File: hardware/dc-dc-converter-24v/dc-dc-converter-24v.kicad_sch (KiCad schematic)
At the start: 56 parts, among them J1 12V, J2 24V, Q1 SQJA42EP, Q2 SQJA42EP, Q3 SQJA42EP, Q4 SQJA42EP, U1 LM5176

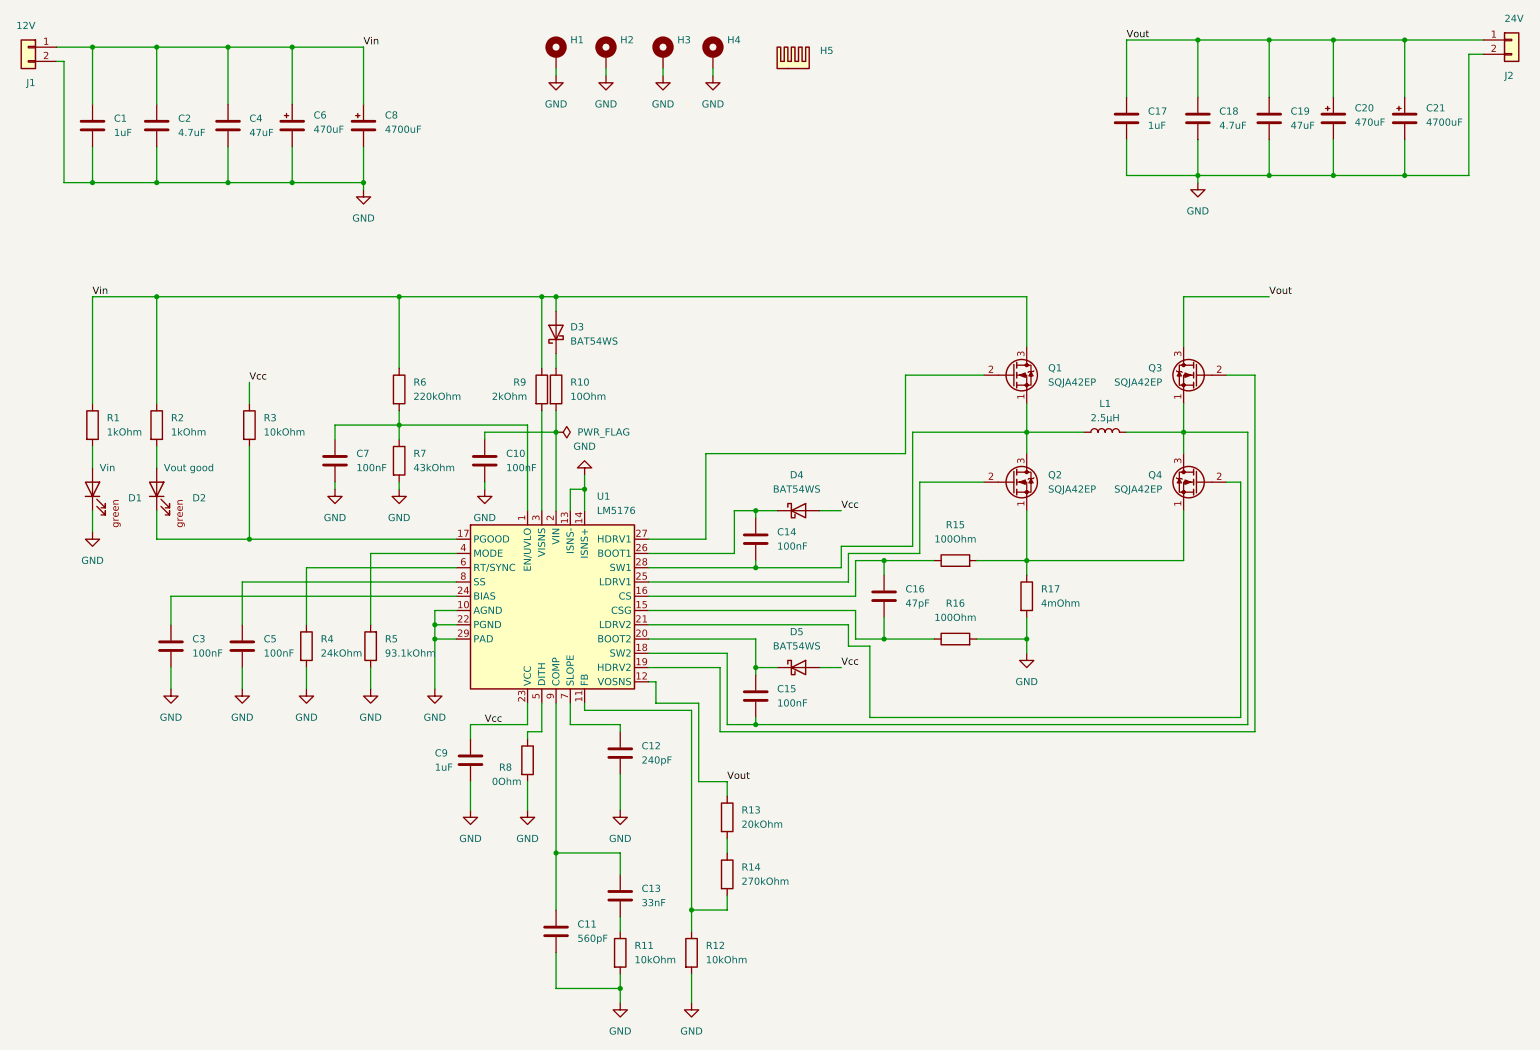
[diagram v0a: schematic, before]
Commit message: start with redesign of DC-DC converter
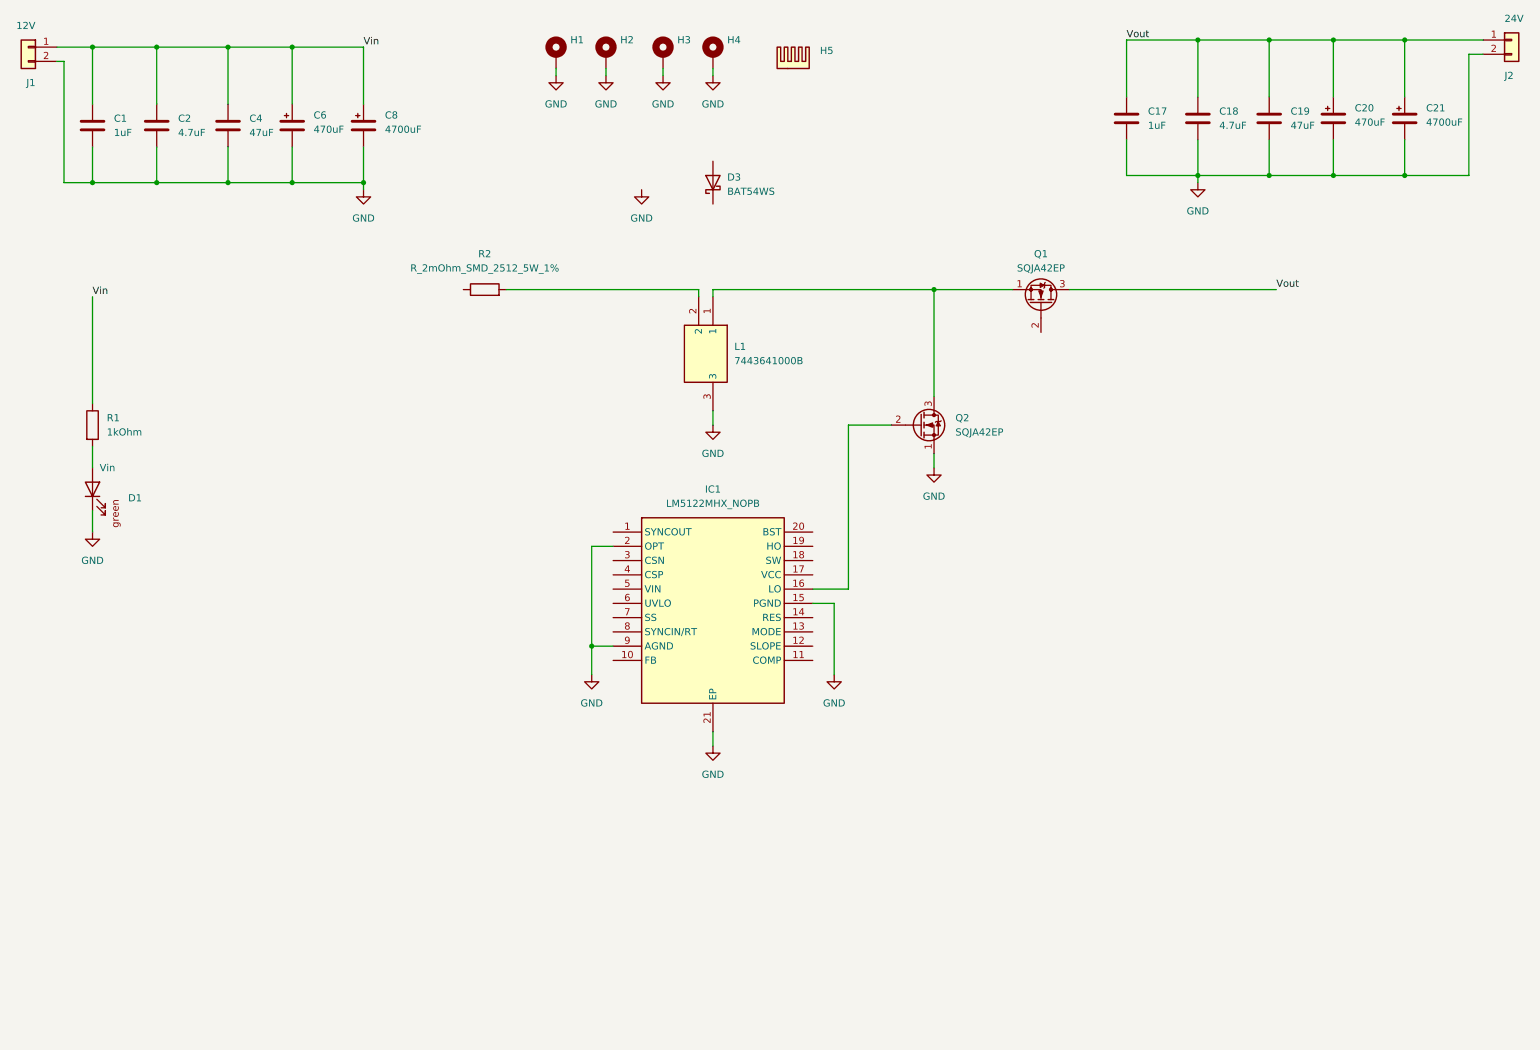
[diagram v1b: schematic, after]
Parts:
- removed C10, C14, C15, C3, C5, C7: 100nF, benediktibk:C_0603_1608Metric_Pad1.08x0.95mm_HandSolder, symbol benediktibk:C_100nF_SMD_0603_50V
- removed C11: 560pF, benediktibk:C_0603_1608Metric_Pad1.08x0.95mm_HandSolder, symbol benediktibk:C_560pF_SMD_0603_50V_5%
- removed C12: 240pF, benediktibk:C_0805_2012Metric_Pad1.18x1.45mm_HandSolder, symbol benediktibk:C_240pF_SMD_0805_250V_10%
- removed C13: 33nF, benediktibk:C_0603_1608Metric_Pad1.08x0.95mm_HandSolder, symbol benediktibk:C_33nF_SMD_0603_50V_10%
- removed C16: 47pF, benediktibk:C_0603_1608Metric_Pad1.08x0.95mm_HandSolder, symbol benediktibk:C_47pF_SMD_0603_100V_5%
- removed C9: 1uF, benediktibk:C_0603_1608Metric_Pad1.08x0.95mm_HandSolder, symbol benediktibk:C_1uF_SMD_0603_50V_10%
- removed D2: Vout good, benediktibk:D_0603_1608Metric_Pad1.05x0.95mm_HandSolder, symbol benediktibk:LED_green_0603
- removed D4, D5: BAT54WS, benediktibk:D_SOD-323, symbol benediktibk:BAT54WS
- removed L1: 2.5µH, benediktibk:ETQP8, symbol benediktibk:L_2_5µH_30A
- removed Q3, Q4: SQJA42EP, benediktibk:SQJA42EPT1_GE3, symbol benediktibk:SQJA42EP
- removed R10: 10Ohm, benediktibk:R_0603_1608Metric_Pad0.98x0.95mm_HandSolder, symbol benediktibk:R_10Ohm_SMD_0603_100mW_1%
- removed R11, R12, R3: 10kOhm, benediktibk:R_0603_1608Metric_Pad0.98x0.95mm_HandSolder, symbol benediktibk:R_10kOhm_SMD_0603_100mW_1%
- removed R13: 20kOhm, benediktibk:R_0603_1608Metric_Pad0.98x0.95mm_HandSolder, symbol benediktibk:R_20kOhm_SMD_0603_100mW_1%
- removed R14: 270kOhm, benediktibk:R_0603_1608Metric_Pad0.98x0.95mm_HandSolder, symbol benediktibk:R_270kOhm_SMD_0603_100mW_1%
- removed R15, R16: 100Ohm, benediktibk:R_0603_1608Metric_Pad0.98x0.95mm_HandSolder, symbol benediktibk:R_100Ohm_SMD_0603_100mW_1%
- removed R17: 4mOhm, benediktibk:R_2512_6332Metric_Pad1.40x3.35mm_HandSolder, symbol benediktibk:R_4mOhm_SMD_2512_2W_1%
- removed R2: 1kOhm, benediktibk:R_0603_1608Metric_Pad0.98x0.95mm_HandSolder, symbol benediktibk:R_1kOhm_SMD_0603_100mW_1%
- removed R4: 24kOhm, benediktibk:R_0603_1608Metric_Pad0.98x0.95mm_HandSolder, symbol benediktibk:R_24kOhm_SMD_0603_100mW_1%
- removed R5: 93.1kOhm, benediktibk:R_0603_1608Metric_Pad0.98x0.95mm_HandSolder, symbol benediktibk:R_93_1kOhm_SMD_0603_100mW_0_1%
- removed R6: 220kOhm, benediktibk:R_0603_1608Metric_Pad0.98x0.95mm_HandSolder, symbol benediktibk:R_220kOhm_SMD_0603_100mW_1%
- removed R7: 43kOhm, benediktibk:R_0603_1608Metric_Pad0.98x0.95mm_HandSolder, symbol benediktibk:R_43kOhm_SMD_0603_100mW_1%
- removed R8: 0Ohm, benediktibk:R_0603_1608Metric_Pad0.98x0.95mm_HandSolder, symbol benediktibk:R_0Ohm_SMD_0603_100mW_0%
- removed R9: 2kOhm, benediktibk:R_0603_1608Metric_Pad0.98x0.95mm_HandSolder, symbol benediktibk:R_2kOhm_SMD_0603_100mW_1%
- removed U1: LM5176, benediktibk:LM5176, symbol benediktibk:LM5176
- added IC1: LM5122MHX_NOPB, benediktibk:SOP65P640X110-21N, symbol benediktibk:LM5122MHX_NOPB
- added L1: 7443641000B, benediktibk:7443641000B, symbol benediktibk:7443641000B
- added R2: R_2mOhm_SMD_2512_5W_1%, benediktibk:R_2512_6332Metric_Pad1.40x3.35mm_HandSolder, symbol benediktibk:R_2mOhm_SMD_2512_5W_1%
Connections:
- net GND: now also Q2.1 (S), IC1.15 (PGND), IC1.2 (OPT), IC1.21 (EP), IC1.9 (AGND), L1.3
- net Vin: no longer D3.2 (A), Q1.3 (D)
- net Vout: now also Q1.3 (D)
- net at Q1.1 (S), Q2.3 (D): now also L1.1
- net at Q2.2 (G): now also IC1.16 (LO)
- new net: L1.2, R2.2
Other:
- moved on the sheet: D3, Q1, Q2
